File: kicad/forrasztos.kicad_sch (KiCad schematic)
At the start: 91 parts, among them J1 24V+-, J2 Conn_02x04_Pin, J3 Conn_01x20_Pin, J4 Conn_01x06_Pin, J5 Conn_02x04_Pin, Q1 AOD409, Q2 MMST2222A, Q3 AOD409, Q4 MMST2222A, SW1 RotaryEncoder_Switch, SW2 SW_Push, SW3 SW_Push, U1 AP63205WU, U2 MCP6004, U3 AP63203WU, U4 24LC00, U5 STM32F103C8Tx, Y1 ATS080B

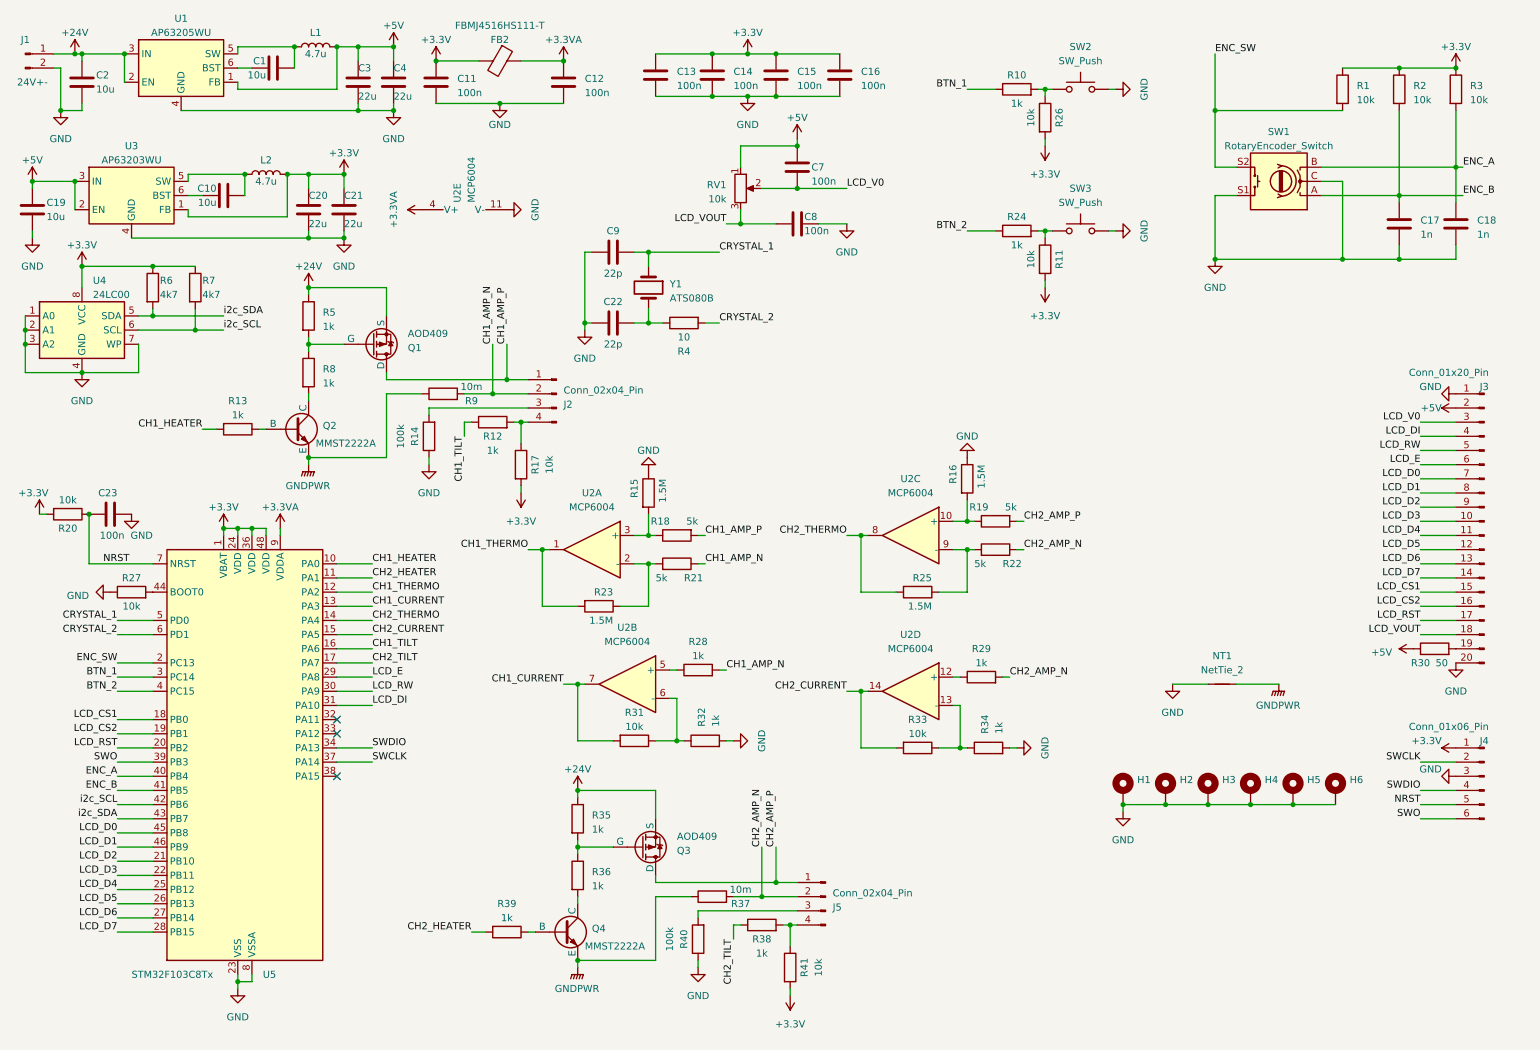
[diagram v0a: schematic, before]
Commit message: hw revision
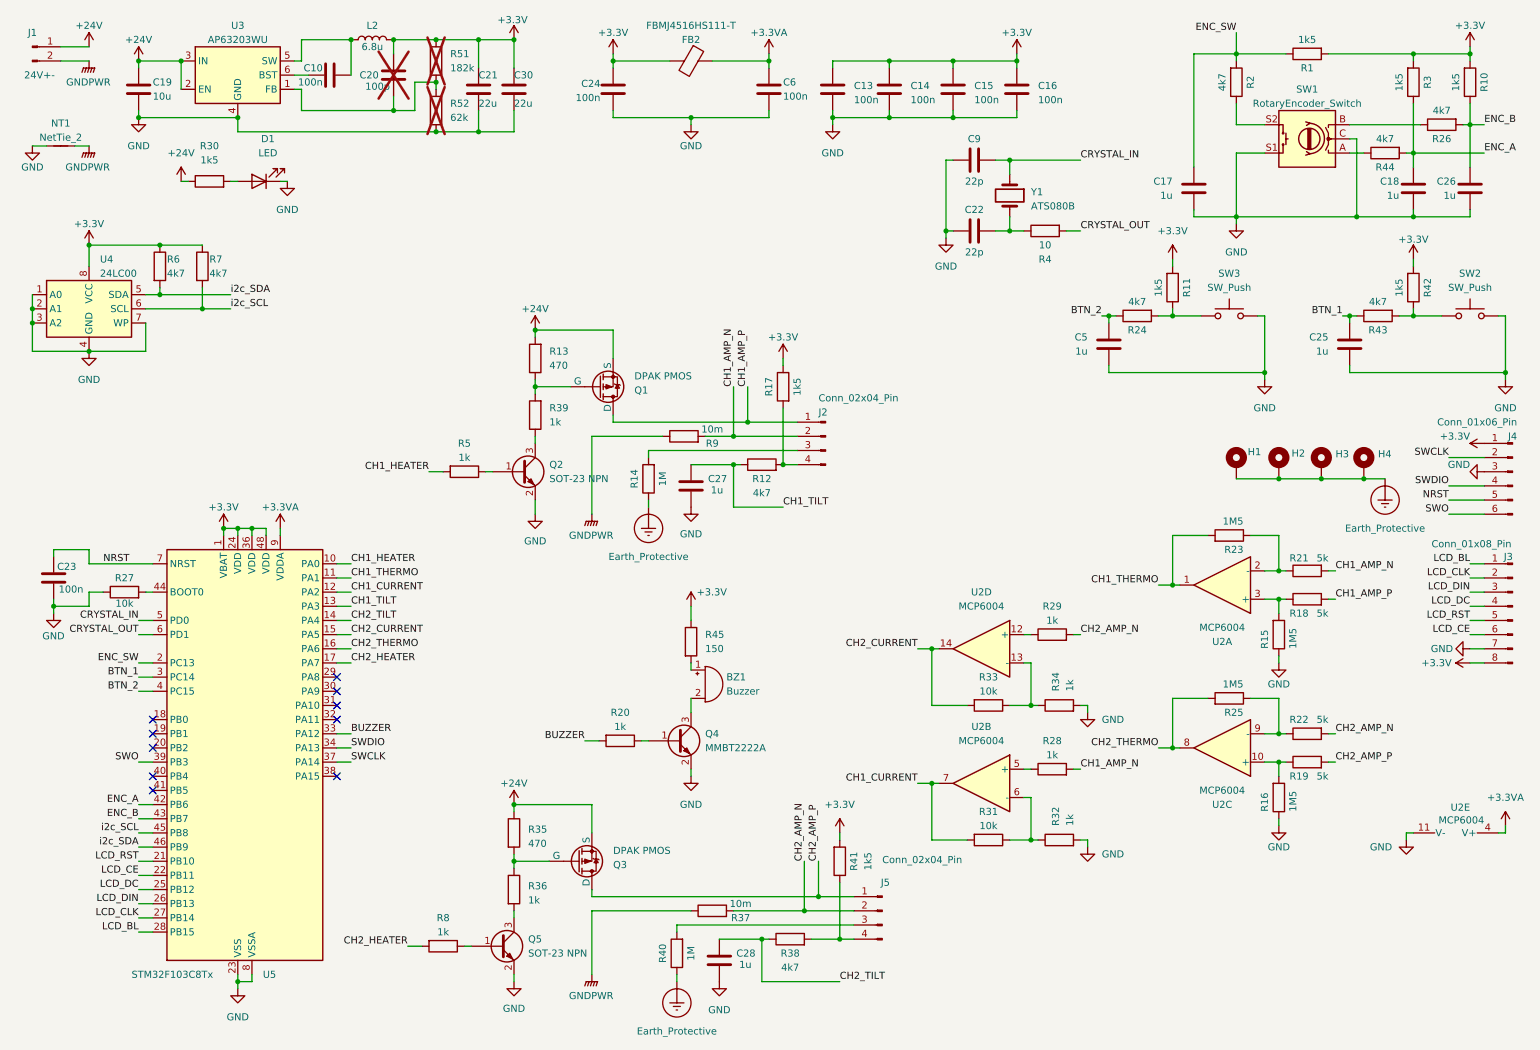
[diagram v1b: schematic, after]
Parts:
- removed C1, C2: 10u, Capacitor_SMD:C_1206_3216Metric_Pad1.33x1.80mm_HandSolder, symbol Device:C
- removed C11, C12, C7, C8: 100n, Capacitor_SMD:C_0805_2012Metric_Pad1.18x1.45mm_HandSolder, symbol Device:C
- removed C3, C4: 22u, Capacitor_SMD:C_1206_3216Metric_Pad1.33x1.80mm_HandSolder, symbol Device:C
- removed H3, H4: MountingHole_Pad, MountingHole:MountingHole_2.5mm_Pad_TopBottom, symbol Mechanical:MountingHole_Pad
- removed J3: Conn_01x20_Pin, Connector_PinHeader_2.54mm:PinHeader_1x20_P2.54mm_Vertical, symbol Connector:Conn_01x20_Pin
- removed L1: 4.7u, Inductor_SMD:L_TracoPower_TCK-047_5.2x5.8mm, symbol Device:L
- removed Q2, Q4: MMST2222A, Package_TO_SOT_SMD:SOT-323_SC-70_Handsoldering, symbol Simulation_SPICE:NPN
- removed RV1: 10k, Potentiometer_SMD:Potentiometer_ACP_CA6-VSMD_Vertical, symbol Device:R_Potentiometer
- removed U1: AP63205WU, Package_TO_SOT_SMD:TSOT-23-6, symbol Regulator_Switching:AP63200WU
- added BZ1: Buzzer, forrasztos_library:BuzzerR9F5, symbol Device:Buzzer
- added C24, C6: 100n, Capacitor_SMD:C_0805_2012Metric_Pad1.18x1.45mm_HandSolder, symbol Device:C
- added C25, C26, C27, C28, C5: 1u, Capacitor_SMD:C_0805_2012Metric_Pad1.18x1.45mm_HandSolder, symbol Device:C
- added C30: 22u, Capacitor_SMD:C_1206_3216Metric_Pad1.33x1.80mm_HandSolder, symbol Device:C
- added D1: LED, LED_SMD:LED_1206_3216Metric_Pad1.42x1.75mm_HandSolder, symbol Device:LED
- added J3: Conn_01x08_Pin, Connector_PinHeader_2.54mm:PinHeader_1x08_P2.54mm_Vertical, symbol Connector:Conn_01x08_Pin
- added Q2, Q5: SOT-23 NPN, Package_TO_SOT_SMD:SOT-323_SC-70_Handsoldering, symbol Transistor_BJT:MMBT2222A
- added Q4: MMBT2222A, Package_TO_SOT_SMD:SOT-323_SC-70_Handsoldering, symbol Transistor_BJT:MMBT2222A
- added R42: 1k5, Resistor_SMD:R_0805_2012Metric_Pad1.20x1.40mm_HandSolder, symbol Device:R
- added R43, R44: 4k7, Resistor_SMD:R_0805_2012Metric_Pad1.20x1.40mm_HandSolder, symbol Device:R
- added R45: 150, Resistor_SMD:R_0805_2012Metric_Pad1.20x1.40mm_HandSolder, symbol Device:R
- added R51: 182k, Resistor_SMD:R_0805_2012Metric_Pad1.20x1.40mm_HandSolder, symbol Device:R
- added R52: 62k, Resistor_SMD:R_0805_2012Metric_Pad1.20x1.40mm_HandSolder, symbol Device:R
- C10: value 10u -> 100n; footprint Capacitor_SMD:C_1206_3216Metric_Pad1.33x1.80mm_HandSolder -> Capacitor_SMD:C_0805_2012Metric_Pad1.18x1.45mm_HandSolder
- C17, C18: value 1n -> 1u
- C20: value 22u -> 100p; footprint Capacitor_SMD:C_1206_3216Metric_Pad1.33x1.80mm_HandSolder -> Capacitor_SMD:C_0805_2012Metric_Pad1.18x1.45mm_HandSolder; now not fitted
- H1: footprint forrasztos_library:MountingHoleOval_3.27x2.5mm -> MountingHole:MountingHole_2.7mm_M2.5_DIN965_Pad_TopBottom
- H2: footprint forrasztos_library:MountingHoleOval_3.27x2.7mm -> MountingHole:MountingHole_2.7mm_M2.5_DIN965_Pad_TopBottom
- H3: renamed from H5; footprint MountingHole:MountingHole_2.5mm_Pad_TopBottom -> MountingHole:MountingHole_2.7mm_M2.5_DIN965_Pad_TopBottom
- H4: renamed from H6; footprint MountingHole:MountingHole_2.5mm_Pad_TopBottom -> MountingHole:MountingHole_2.7mm_M2.5_DIN965_Pad_TopBottom
- L2: value 4.7u -> 6.8u
- NT1: footprint NetTie:NetTie-2_SMD_Pad0.5mm -> NetTie:NetTie-2_SMD_Pad2.0mm
- Q1, Q3: value AOD409 -> DPAK PMOS
- R1, R11, R17, R3, R41: value 10k -> 1k5
- R10: value 1k -> 1k5
- R12, R24, R38: value 1k -> 4k7
- R13, R35: value 1k -> 470
- R14, R40: value 100k -> 1M; footprint Resistor_THT:R_Axial_DIN0207_L6.3mm_D2.5mm_P10.16mm_Horizontal -> Resistor_THT:R_Axial_DIN0414_L11.9mm_D4.5mm_P15.24mm_Horizontal
- R15, R16, R23, R25: value 1.5M -> 1M5
- R2, R26: value 10k -> 4k7
- R20: value 10k -> 1k
- R30: value 50 -> 1k5; footprint Resistor_THT:R_Axial_DIN0207_L6.3mm_D2.5mm_P10.16mm_Horizontal -> Resistor_SMD:R_0805_2012Metric_Pad1.20x1.40mm_HandSolder
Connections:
- net +5V is gone; now on net +24V: C19.1, R30.1, U3.2 (EN), U3.3 (IN)
- net LCD_D0 is gone; now on net i2c_SCL: U5.45 (PB8)
- net LCD_D1 is gone; now on net i2c_SDA: U5.46 (PB9)
- net LCD_D2 is gone; now on net LCD_RST: U5.21 (PB10)
- net +24V: now also R13.2; no longer R5.1
- net +3.3V: now also R1.2, R10.2, R17.1, R3.2, C24.1, C30.1, J3.8 (Pin_8), R42.2, R45.1, R51.1; no longer R1.1, R17.2, R2.1, R20.2, R26.2, R3.1, U3.1 (FB)
- net +3.3VA: now also C6.1
- net BTN_1: now also C25.1, R43.1; no longer R10.1
- net BTN_2: now also C5.1
- net CH1_AMP_N: now also R21.2; no longer R21.1
- net CH1_CURRENT: now also U5.12 (PA2); no longer U5.13 (PA3)
- net CH1_HEATER: now also R5.2; no longer R13.2
- net CH1_THERMO: now also U5.11 (PA1); no longer U5.12 (PA2)
- net CH1_TILT: now also U5.13 (PA3), C27.2; no longer U5.16 (PA6)
- net CH2_AMP_N: now also R22.2; no longer R22.1
- net CH2_HEATER: now also R8.2, U5.17 (PA7); no longer R39.2, U5.11 (PA1)
- net CH2_THERMO: now also U5.16 (PA6); no longer U5.14 (PA4)
- net CH2_TILT: now also U5.14 (PA4), C28.2; no longer U5.17 (PA7)
- net ENC_A: now also R3.1, U5.42 (PB6), R44.2; no longer R3.2, SW1.B, U5.40 (PB4)
- net ENC_B: now also R10.1, R26.2, U5.43 (PB7), C26.1; no longer C17.1, R2.2, SW1.A, U5.41 (PB5)
- net ENC_SW: now also C17.1, R1.1, R2.2; no longer R1.2, SW1.S2
- net GND: now also C23.1, C24.2, C25.2, C26.2, C27.1, C28.1, C30.2, C5.2, C6.2, D1.1 (K), J3.7 (Pin_7), Q2.2 (E), Q4.2 (E), Q5.2 (E), R52.2; no longer C20.2, C23.2, H1.1, H2.1, H3.1, H4.1, J1.2 (Pin_2), R14.1, R40.1
- net GNDPWR: now also J1.2 (Pin_2)
- net LCD_RST: now also J3.5 (Pin_5); no longer U5.20 (PB2)
- net NRST: now also C23.2; no longer C23.1, R20.1
- net i2c_SCL: no longer U5.42 (PB6)
- net i2c_SDA: no longer U5.43 (PB7)
- net at R30.2: now also D1.2 (A)
- net at R13.1: now also Q1.2 (G), R39.2
- net BUZZER: now reaches U5.33 (PA12)
- net BUZZER: now also R20.2
- net at R39.1: now also Q2.3 (C)
- net at R36.2: now also Q5.3 (C)
- net at R25.1, U2.9 (-): now also R22.1; no longer R22.2
- net at R23.1, U2.2 (-): now also R21.1; no longer R21.2
- net at J2.4 (Pin_4), R12.2: now also R17.2; no longer R17.1
- net CRYSTAL_1 renamed CRYSTAL_IN
- net CRYSTAL_2 renamed CRYSTAL_OUT
- net LCD_CS1: no longer names the net of U5.18 (PB0)
- net LCD_CS2: no longer names the net of U5.19 (PB1)
- net LCD_D3 renamed LCD_CE
- net LCD_CE: now also J3.6 (Pin_6)
- net LCD_D4 renamed LCD_DC
- net LCD_DC: now also J3.4 (Pin_4)
- net LCD_D5 renamed LCD_DIN
- net LCD_DIN: now also J3.3 (Pin_3)
- net LCD_D6 renamed LCD_CLK
- net LCD_CLK: now also J3.2 (Pin_2)
- net LCD_D7 renamed LCD_BL
- net LCD_BL: now also J3.1 (Pin_1)
- net LCD_DI: no longer names the net of U5.31 (PA10)
- net LCD_E: no longer names the net of U5.29 (PA8)
- net LCD_RW: no longer names the net of U5.30 (PA9)
- new net: R44.1, SW1.A
- new net: R2.1, SW1.S2
- new net: BZ1.1 (+), R45.2
- new net: R42.1, R43.2, SW2.1
- new net: C20.2, R51.2, R52.1, U3.1 (FB)
- new net: Q2.1 (B), R5.1
- new net: Q4.1 (B), R20.1
- new net: BZ1.2 (-), Q4.3 (C)
- new net: R26.1, SW1.B
- new net: Q5.1 (B), R8.1
- new net Earth_Protective: H1.1, H2.1, H3.1, H4.1, R14.1, R40.1
- no-connect marks 3 -> 10
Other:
- moved on the sheet: C13, C14, C15, C16, C19, C22, C23, C9, FB2, H3, H4, J2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

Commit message: flip led
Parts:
- D1: footprint LED_SMD:LED_1206_3216Metric_Pad1.42x1.75mm_HandSolder -> LED_THT:LED_D3.0mm
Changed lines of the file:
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@@
 			)
 		)
-		(property "Footprint" "LED_SMD:LED_1206_3216Metric_Pad1.42x1.75mm_HandSolder"
+		(property "Footprint" "LED_THT:LED_D3.0mm"
 			(at 57.15 43.18 0)
 			(effects
